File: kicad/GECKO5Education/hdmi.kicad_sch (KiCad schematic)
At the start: 10 parts, among them J2 HDMI_A, J6 Conn_01x06_Socket, J7 Conn_01x02_Pin, U16 LTC2632CTS8-LZ12TRMPBF, U17 MAX11666AUBV, U3 SII9022ACNU, U6 LFE5U-85F-6BG381x

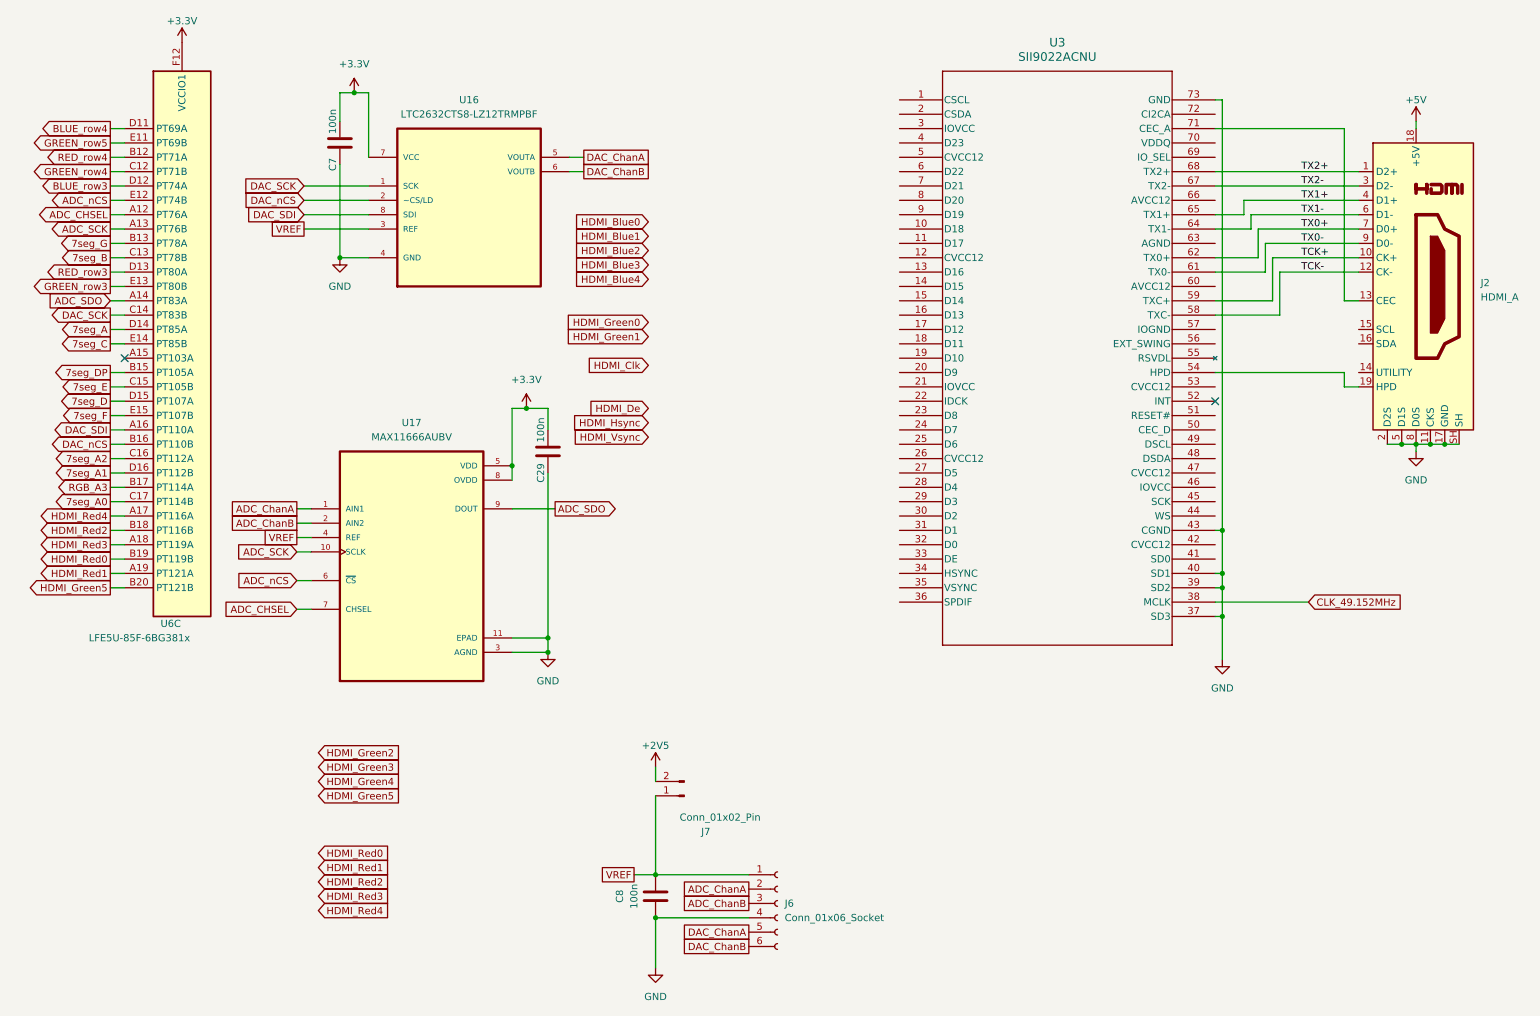
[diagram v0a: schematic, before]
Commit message: Added SII9022
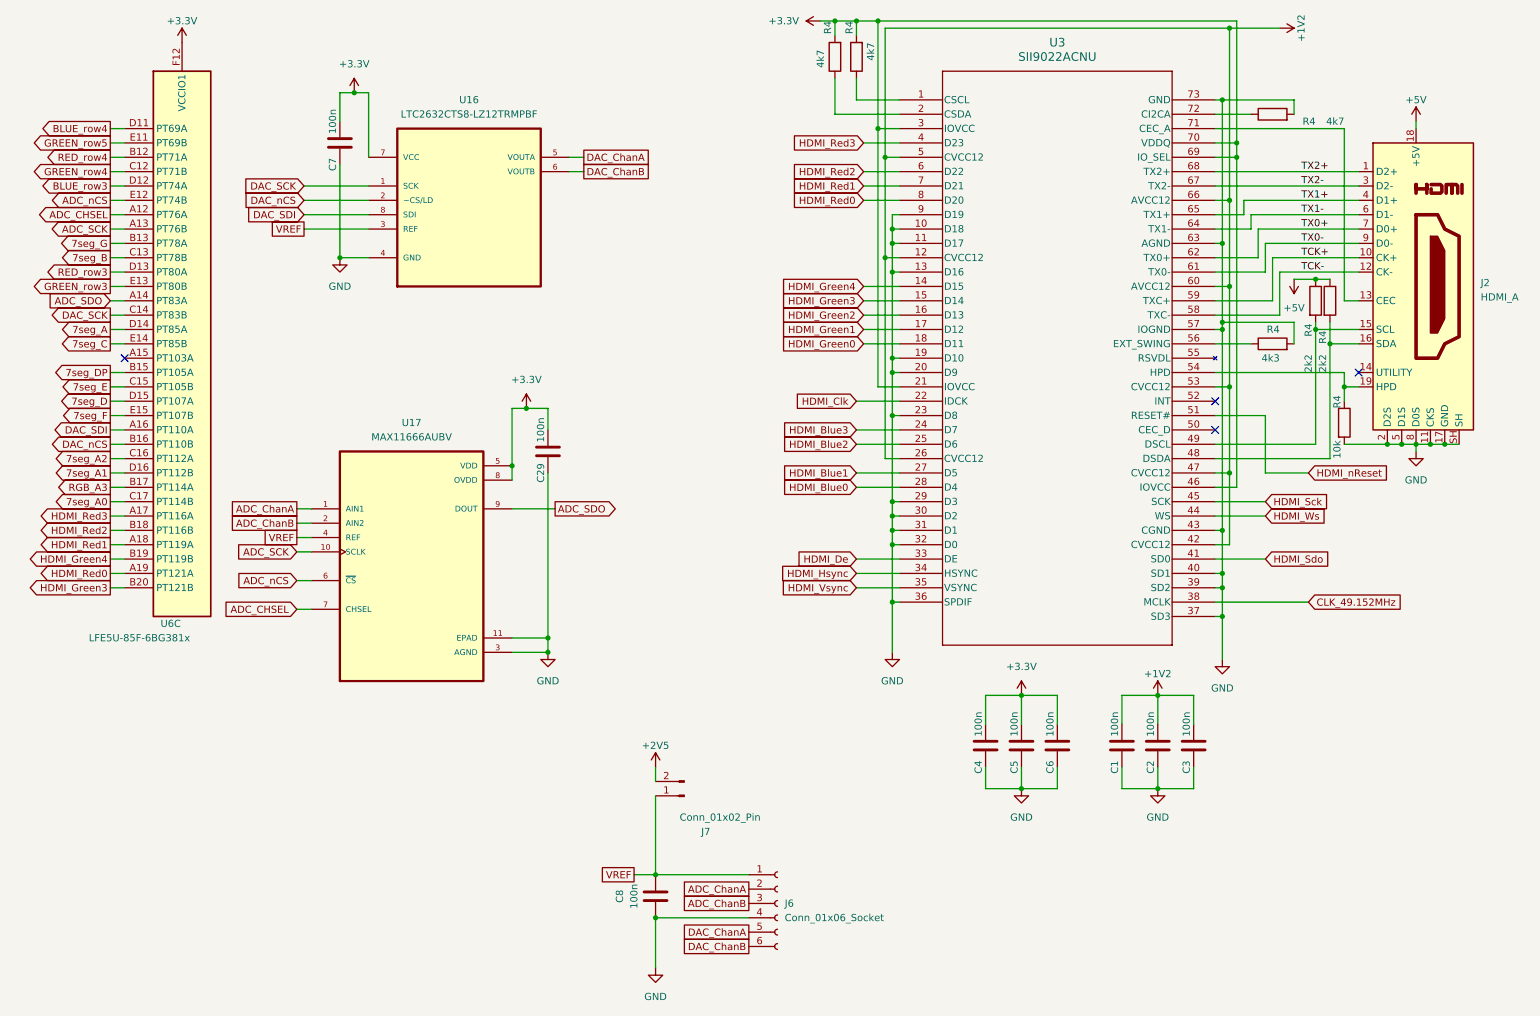
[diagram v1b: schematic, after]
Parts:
- added C1, C2, C3, C4, C5, C6: 100n, Resistor_SMD:R_0402_1005Metric, symbol Device:C
- added R4 (x3): 4k7, Resistor_SMD:R_0402_1005Metric, symbol Device:R
- added R4 (x2): 2k2, Resistor_SMD:R_0402_1005Metric, symbol Device:R
- added R4: 4k3, Resistor_SMD:R_0402_1005Metric, symbol Device:R
- added R4: 10k, Resistor_SMD:R_0402_1005Metric, symbol Device:R
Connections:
- net HDMI_Green5 is gone; now on net HDMI_Green3: U6.B20 (PT121B)
- net HDMI_Red4 is gone; now on net HDMI_Red3: U6.A17 (PT116A)
- net +3.3V: now also U3.21 (IOVCC), U3.3 (IOVCC), U3.46 (IOVCC), U3.69 (IO_SEL), U3.70 (VDDQ), C4.2, C5.2, C6.2, R4.2, R4.2
- net +5V: now also R4.1, R4.1
- net GND: now also U3.10 (D18), U3.11 (D17), U3.13 (D16), U3.19 (D10), U3.20 (D9), U3.23 (D8), U3.29 (D3), U3.30 (D2), U3.31 (D1), U3.32 (D0), U3.36 (SPDIF), U3.57 (IOGND), U3.63 (AGND), U3.9 (D19), C1.1, C2.1, C3.1, C4.1, C5.1, C6.1, R4.2, R4.2, R4.2
- net HDMI_Blue0: now also U3.28 (D4)
- net HDMI_Blue1: now also U3.27 (D5)
- net HDMI_Blue2: now also U3.25 (D6)
- net HDMI_Blue3: now also U3.24 (D7)
- net HDMI_Clk: now also U3.22 (IDCK)
- net HDMI_De: now also U3.33 (DE)
- net HDMI_Green0: now also U3.18 (D11)
- net HDMI_Green1: now also U3.17 (D12)
- net HDMI_Green2: now also U3.16 (D13)
- net HDMI_Green3: now also U3.15 (D14)
- net HDMI_Green4: now also U3.14 (D15), U6.B19 (PT119B)
- net HDMI_Hsync: now also U3.34 (HSYNC)
- net HDMI_Red0: now also U3.8 (D20), U6.A19 (PT121A); no longer U6.B19 (PT119B)
- net HDMI_Red1: now also U3.7 (D21), U6.A18 (PT119A); no longer U6.A19 (PT121A)
- net HDMI_Red2: now also U3.6 (D22)
- net HDMI_Red3: now also U3.4 (D23); no longer U6.A18 (PT119A)
- net HDMI_Vsync: now also U3.35 (VSYNC)
- net at J2.15 (SCL): now also U3.49 (DSCL), R4.2
- net at J2.16 (SDA): now also U3.48 (DSDA), R4.2
- net at J2.19 (HPD), U3.54 (HPD): now also R4.1
- net at U3.1 (CSCL): now also R4.1
- net +1V2: now reaches U3.12 (CVCC12)
- net +1V2: now also U3.26 (CVCC12), U3.42 (CVCC12), U3.47 (CVCC12), U3.5 (CVCC12), U3.53 (CVCC12), U3.60 (AVCC12), U3.66 (AVCC12), C1.2, C2.2, C3.2
- net at U3.2 (CSDA): now also R4.1
- net HDMI_Sdo: now reaches U3.41 (SD0)
- net HDMI_Ws: now reaches U3.44 (WS)
- net HDMI_Sck: now reaches U3.45 (SCK)
- net HDMI_nReset: now reaches U3.51 (RESET#)
- net at U3.56 (EXT_SWING): now also R4.1
- net at U3.72 (CI2CA): now also R4.1
- no-connect marks 2 -> 4
